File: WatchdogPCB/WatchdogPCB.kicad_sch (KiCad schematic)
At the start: 18 parts, among them J1 Screw_Terminal_01x03, J2 Screw_Terminal_01x04, J3 Screw_Terminal_01x02, J4 Conn_01x05_Pin, U1 MCP602, U2 A1301EUA-T, U3 DS3695N

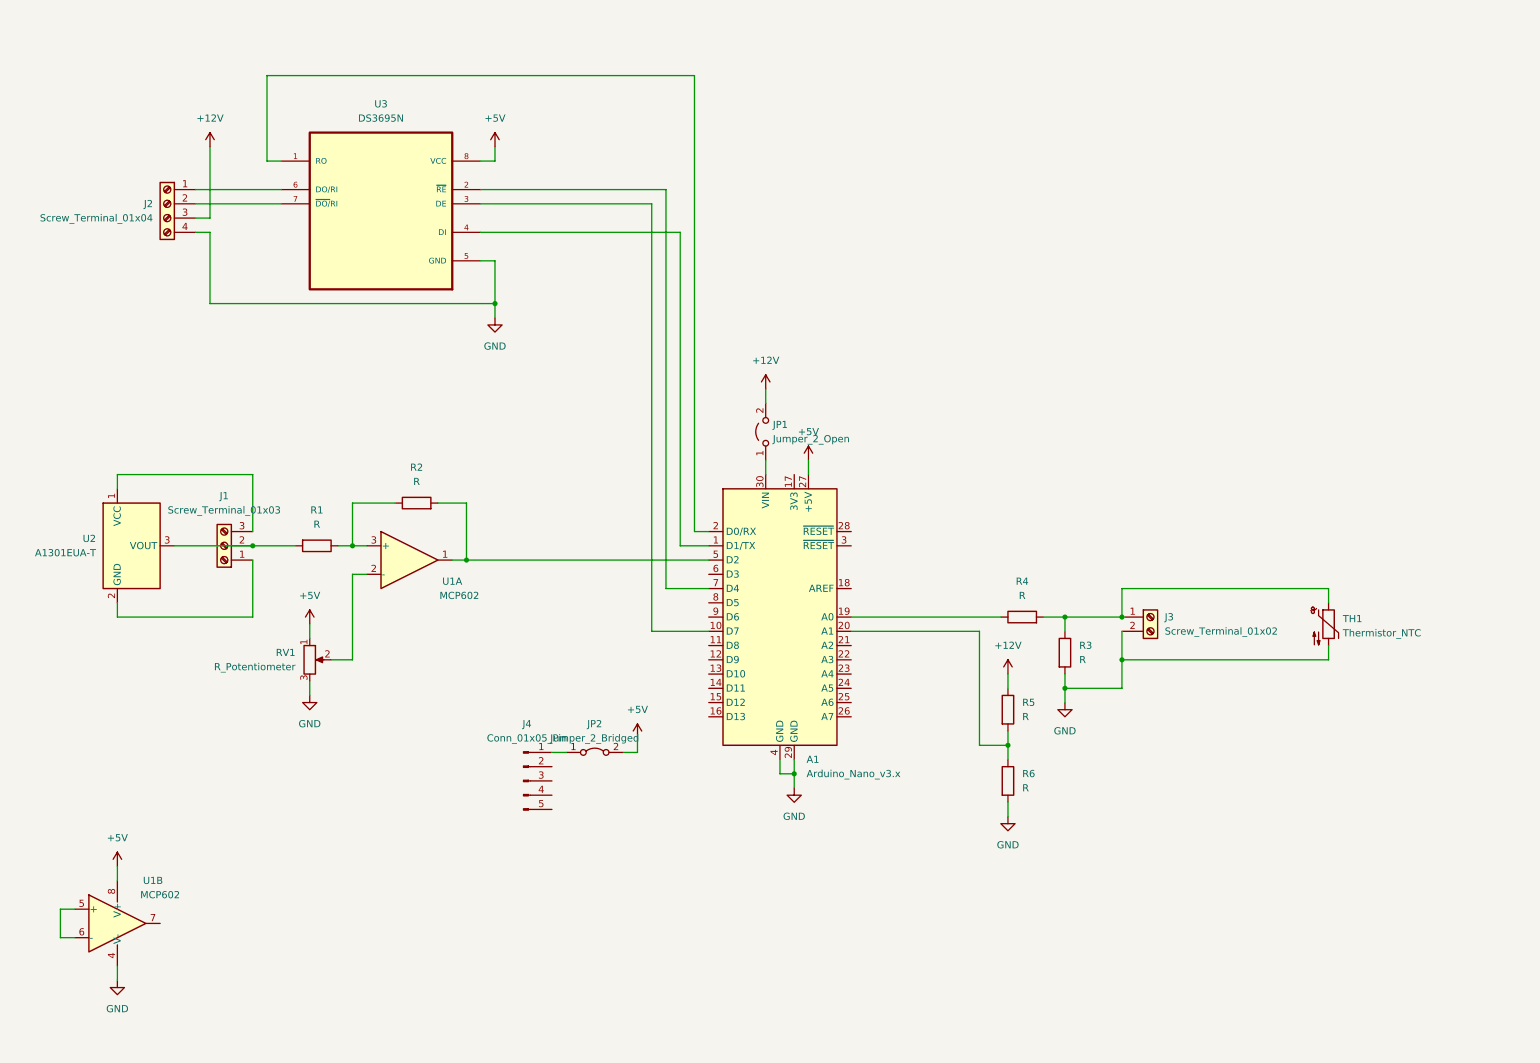
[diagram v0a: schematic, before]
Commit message: Schematic finished
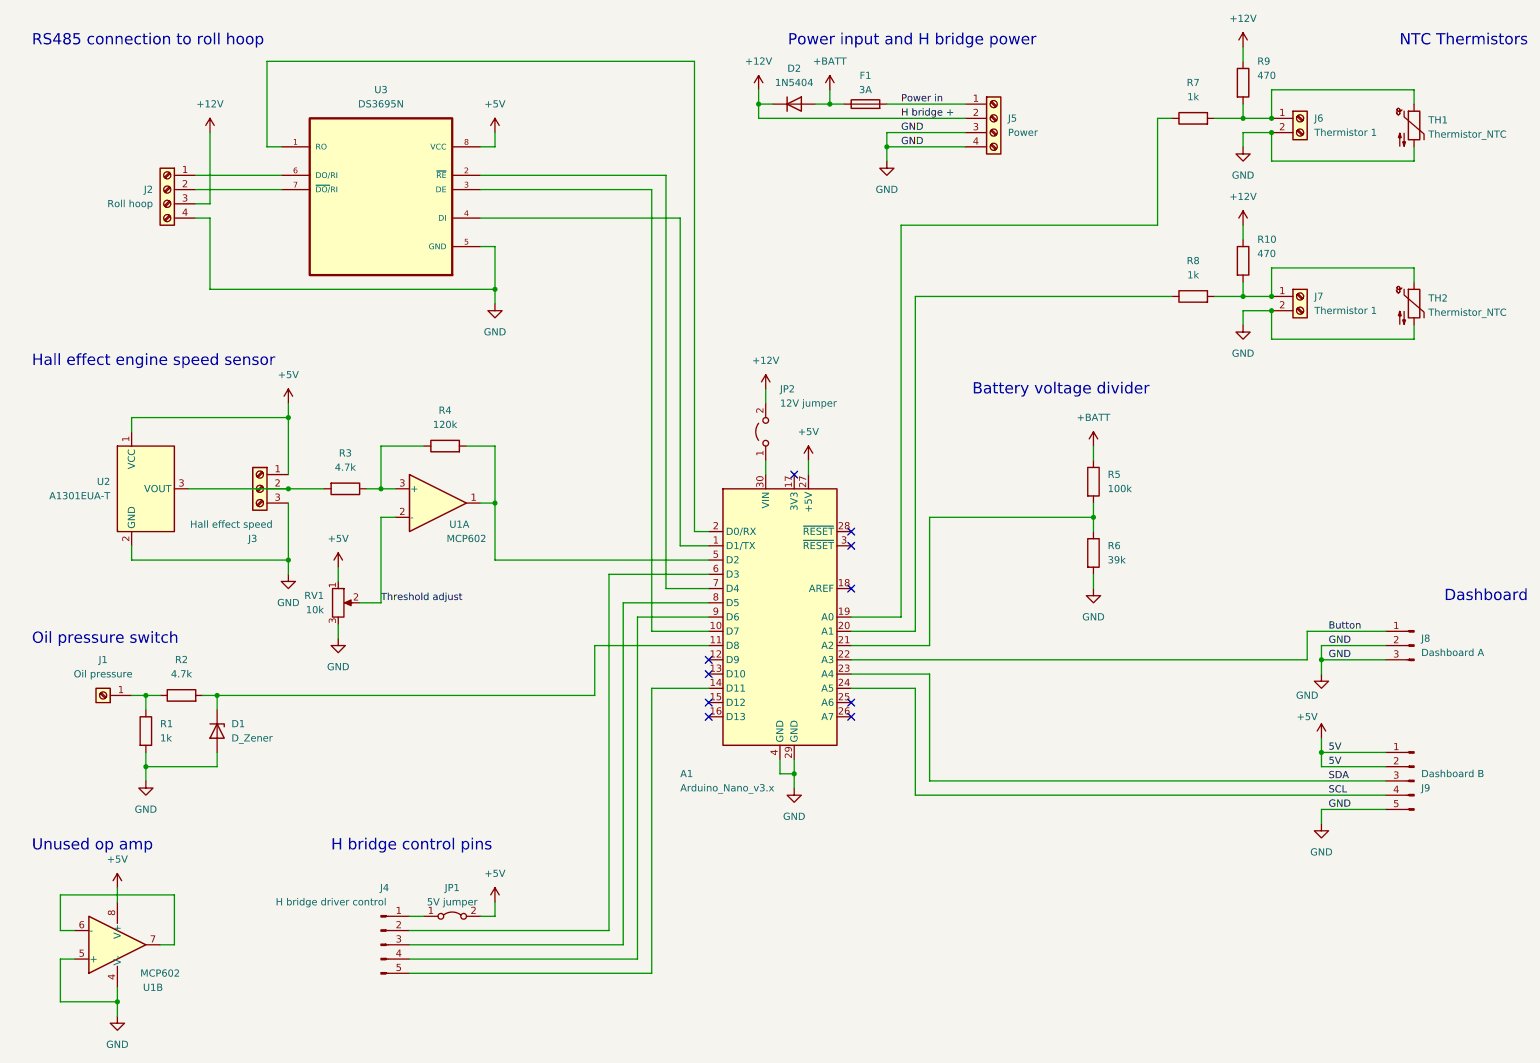
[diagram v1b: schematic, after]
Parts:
- removed J1: Screw_Terminal_01x03, symbol Connector:Screw_Terminal_01x03
- removed J3: Screw_Terminal_01x02, symbol Connector:Screw_Terminal_01x02
- removed R3, R4: R, symbol Device:R
- added D1: D_Zener, symbol Device:D_Zener
- added D2: 1N5404, Diode_THT:D_DO-201AD_P15.24mm_Horizontal, symbol Diode:1N5404
- added F1: 3A, symbol Device:Fuse
- added J1: Oil pressure, symbol Connector:Screw_Terminal_01x01
- added J3: Hall effect speed, symbol Connector:Screw_Terminal_01x03
- added J5: Power, symbol Connector:Screw_Terminal_01x04
- added J6, J7: Thermistor 1, symbol Connector:Screw_Terminal_01x02
- added J8: Dashboard A, symbol Connector:Conn_01x03_Pin
- added J9: Dashboard B, symbol Connector:Conn_01x05_Pin
- added R1, R7, R8: 1k, symbol Device:R
- added R10, R9: 470, symbol Device:R
- added R2: 4.7k, symbol Device:R
- added TH2: Thermistor_NTC, symbol Device:Thermistor_NTC
- J2: value Screw_Terminal_01x04 -> Roll hoop
- J4: value Conn_01x05_Pin -> H bridge driver control
- JP1: renamed from JP2; value Jumper_2_Bridged -> 5V jumper
- JP2: renamed from JP1; value Jumper_2_Open -> 12V jumper
- R3: renamed from R1; value R -> 4.7k
- R4: renamed from R2; value R -> 120k
- R5: value R -> 100k
- R6: value R -> 39k
- RV1: value R_Potentiometer -> 10k
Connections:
- net +12V: now also D2.1 (K), J5.2 (Pin_2), R10.1, R9.1; no longer R5.1
- net +5V: now also U2.1 (VCC), J3.1 (Pin_1), J9.1 (Pin_1), J9.2 (Pin_2)
- net GND: now also U1.5 (+), U2.2 (GND), D1.2 (A), J3.3 (Pin_3), J5.3 (Pin_3), J5.4 (Pin_4), J6.2 (Pin_2), J7.2 (Pin_2), J8.2 (Pin_2), J8.3 (Pin_3), J9.5 (Pin_5), R1.2, TH2.2
- net at A1.19 (A0): now also R7.1
- net at TH1.1: now also J6.1 (Pin_1), R7.2, R9.2
- net at A1.11 (D8): now also D1.1 (K), R2.2
- net at A1.14 (D11): now also J4.5 (Pin_5)
- net at R5.2, R6.1: now also A1.21 (A2); no longer A1.20 (A1)
- net Button: now reaches A1.22 (A3)
- net Button: now also J8.1 (Pin_1)
- net SDA: now reaches A1.23 (A4)
- net SDA: now also J9.3 (Pin_3)
- net SCL: now reaches A1.24 (A5)
- net SCL: now also J9.4 (Pin_4)
- net at A1.6 (D3): now also J4.2 (Pin_2)
- net at A1.8 (D5): now also J4.3 (Pin_3)
- net at A1.9 (D6): now also J4.4 (Pin_4)
- net at U1.6 (-): now also U1.7; no longer U1.5 (+)
- net at R3.2, U2.3 (VOUT): now also J3.2 (Pin_2)
- net Threshold adjust: now reaches RV1.2, U1.2 (-)
- new net: J7.1 (Pin_1), R10.2, R8.2, TH2.1
- new net: A1.20 (A1), R8.1
- new net: J1.1 (Pin_1), R1.1, R2.1
- new net +BATT: D2.2 (A), F1.1, R5.1
- new net Power in: F1.2, J5.1 (Pin_1)
- no-connect marks 0 -> 10
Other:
- note added: "Battery voltage divider"
- note added: "Dashboard"
- note added: "H bridge control pins"
- note added: "Hall effect engine speed sensor"
- note added: "NTC Thermistors"
- note added: "Oil pressure switch"
- note added: "Power input and H bridge power"
- note added: "RS485 connection to roll hoop"
- note added: "Unused op amp"
- moved on the sheet: J2, J4, JP1, R3, R4, R5, R6, RV1, U1A, U1B, U2, U3
